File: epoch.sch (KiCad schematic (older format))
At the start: 26 parts, among them P1 USB_OTG, P3 CONN_01X10, P4 CONN_02X05, SW1 SW_Reset, SW2 SW_Up, SW3 SW_Middle, SW4 SW_Down, U1 MIC5219-3.3BM5, U2 ATSAMD21Ennc-AU, U3 DS3231MZ, U5 74HC1G14GW, Y1 32.768kHz

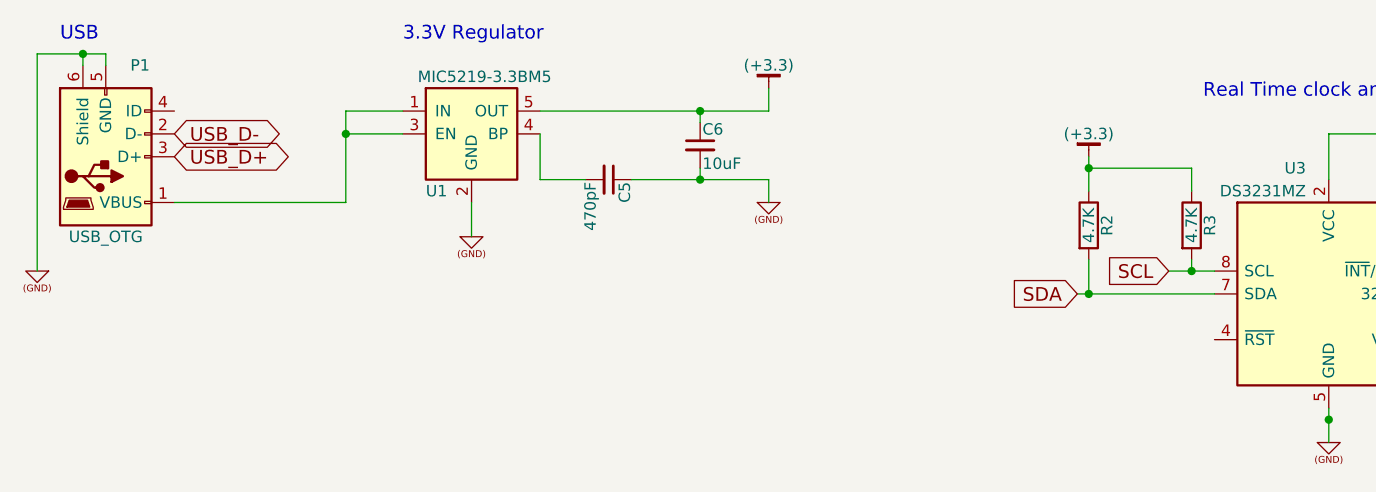
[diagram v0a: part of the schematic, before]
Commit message: More Layout
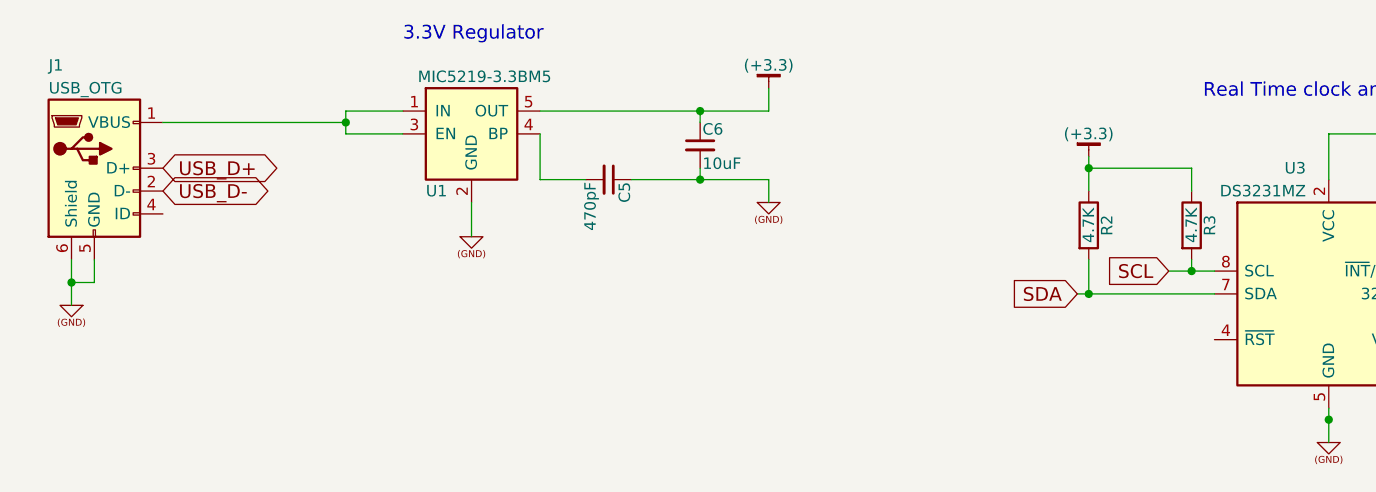
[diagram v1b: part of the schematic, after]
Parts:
- removed P1: USB_OTG, Connectors_Molex:USB_Micro-B_Molex_47346-0001, symbol USB_OTG
- added J1: USB_OTG, Connectors:USB-MICROB_LARGEPAD, symbol USB_OTG
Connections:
- net (GND): now also J1.5 (GND), J1.6 (Shield)
- net USB_D+: now also J1.3 (D+)
- net USB_D-: now also J1.2 (D-)
- net at U1.1 (IN), U1.3 (EN): now also J1.1 (VBUS)
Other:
- note removed: "USB"
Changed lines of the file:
@@
 RESET
-$Comp
-L USB_OTG P1
-U 1 1 58B3A824
-P 1750 1350
-F 0 "P1" H 1900 950 50  0000 C CNN
-F 1 "USB_OTG" H 1750 1700 50  0000 C CNN
-F 2 "Connectors_Molex:USB_Micro-B_Molex_47346-0001" V 1700 1250 50  0001 C CNN
-F 3 "" V 1700 1250 50  0000 C CNN
-	1    1750 1350
-	1    0    0    1
-$EndComp
 $Comp
 L (GND) #PWR010
 U 1 1 58B3A991
-P 1450 1850
-F 0 "#PWR010" H 1450 1850 30  0001 C CNN
-F 1 "(GND)" H 1450 1850 30  0001 C CNN
-F 2 "" H 1450 1850 60  0000 C CNN
-F 3 "" H 1450 1850 60  0000 C CNN
-	1    1450 1850
+P 1600 2000
+F 0 "#PWR010" H 1600 2000 30  0001 C CNN
+F 1 "(GND)" H 1600 2000 30  0001 C CNN
+F 2 "" H 1600 2000 60  0000 C CNN
+F 3 "" H 1600 2000 60  0000 C CNN
+	1    1600 2000
 	-1   0    0    -1
 $EndComp
-Text GLabel 2050 1250 2    60   BiDi ~ 0
+Text GLabel 2000 1500 2    60   BiDi ~ 0
 USB_D-
-Text GLabel 2050 1350 2    60   BiDi ~ 0
+Text GLabel 2000 1400 2    60   BiDi ~ 0
 USB_D+
 $Comp
@@
 	1    0    0    -1
 $EndComp
-Wire Wire Line
-	2800 1250 3050 1250
 $Comp
 L (GND) #PWR011
@@
 Wire Wire Line
 	4350 1150 4350 1200
-Text Notes 1550 850  0    60   ~ 0
-USB
 Text Notes 3050 850  0    60   ~ 0
 3.3V Regulator
@@
 	8500 2150 8500 2600
 Wire Wire Line
-	1650 950  1650 900
-Wire Wire Line
-	1450 900  1750 900
-Wire Wire Line
-	1450 900  1450 1850
-Wire Wire Line
-	1750 900  1750 950
-Connection ~ 1650 900
-Wire Wire Line
-	2800 1550 2050 1550
-Wire Wire Line
-	2800 1150 2800 1550
+	2800 1150 2800 1250
 Wire Wire Line
 	2800 1150 3050 1150
-Connection ~ 2800 1250
+Connection ~ 2800 1200
 $Comp
 L SW_Push SW2
@@
 SDA
 Wire Wire Line
-	6600 1850 6400 1850
-Wire Wire Line
-	6600 1950 6000 1950
+	6400 1850 6600 1850
+Wire Wire Line
+	6000 1950 6600 1950
 $Comp
 L R R3
@@
 Connection ~ 6050 1950
 Wire Wire Line
-	6050 1500 6050 1350
+	6050 1350 6050 1500
 Wire Wire Line
 	6500 1850 6500 1800
@@
 Text GLabel 3750 4600 2    60   Input ~ 0
 BUT_UP
+$Comp
+L USB_OTG J1
+U 1 1 58F5A24A
+P 1700 1400
+F 0 "J1" H 1500 1850 50  0000 L CNN
+F 1 "USB_OTG" H 1500 1750 50  0000 L CNN
+F 2 "Connectors:USB-MICROB_LARGEPAD" H 1850 1350 50  0001 C CNN
+F 3 "" H 1850 1350 50  0001 C CNN
+	1    1700 1400
+	1    0    0    -1
+$EndComp
+Wire Wire Line
+	2800 1250 3050 1250
+Wire Wire Line
+	1600 1800 1600 2000
+Wire Wire Line
+	1700 1800 1700 1900
+Wire Wire Line
+	1700 1900 1600 1900
+Connection ~ 1600 1900
+Wire Wire Line
+	2000 1200 2800 1200
 $EndSCHEMATC
